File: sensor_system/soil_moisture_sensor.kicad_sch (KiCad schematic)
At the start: 15 parts, among them U1 TLC555xD, U2 XC6206PxxxMR

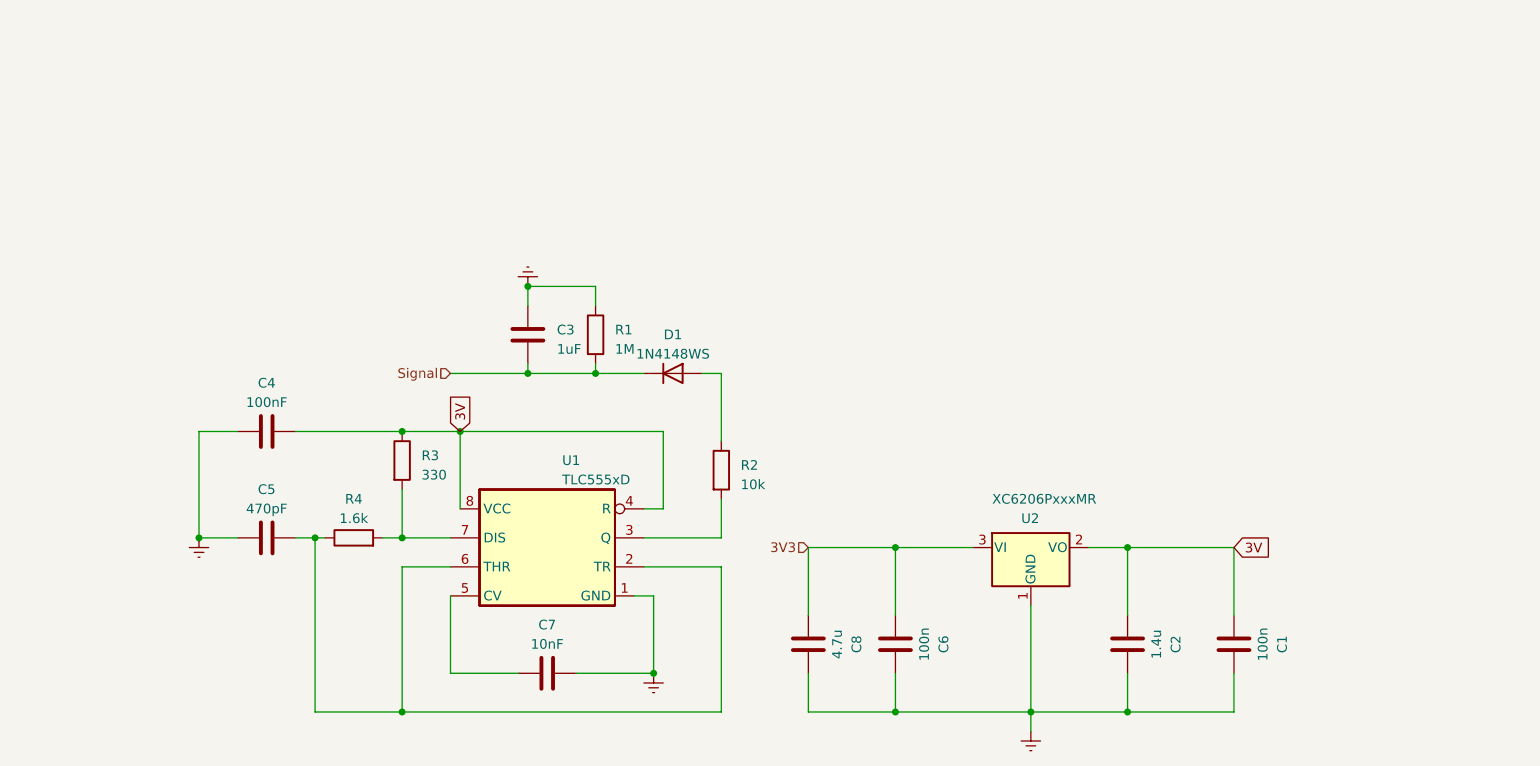
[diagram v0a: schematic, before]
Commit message: Gala versija
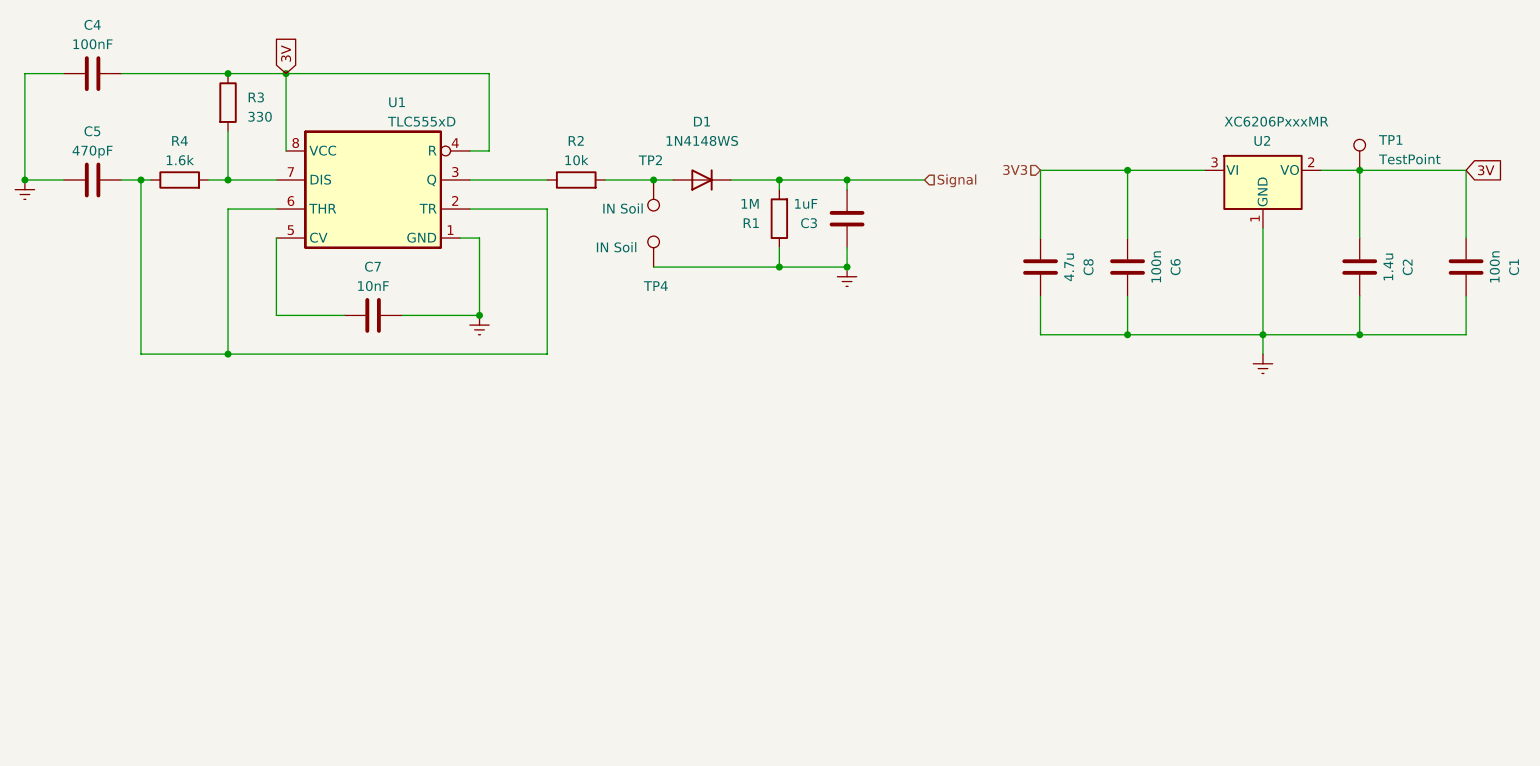
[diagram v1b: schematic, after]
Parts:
- added TP1: TestPoint, Connector_PinHeader_1.00mm:PinHeader_1x01_P1.00mm_Vertical, symbol Connector:TestPoint
- added TP2, TP4: IN Soil, symbol Connector:TestPoint
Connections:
- net 3V: now also TP1.1
- net Earth: now also TP4.1
- net at U1.3 (Q): now also R2.1; no longer R2.2
- net at D1.2 (A): now also R2.2, TP2.1; no longer R2.1
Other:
- moved on the sheet: C1, C2, C3, C4, C5, C6, C7, C8, D1, R1, R2, R3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
